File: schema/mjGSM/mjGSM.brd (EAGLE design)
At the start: 62 x 47 mm, 20 parts, among them Q1 16MHz, SW1 SPST, U1 ATMEGA328P-PU, X2 PWR

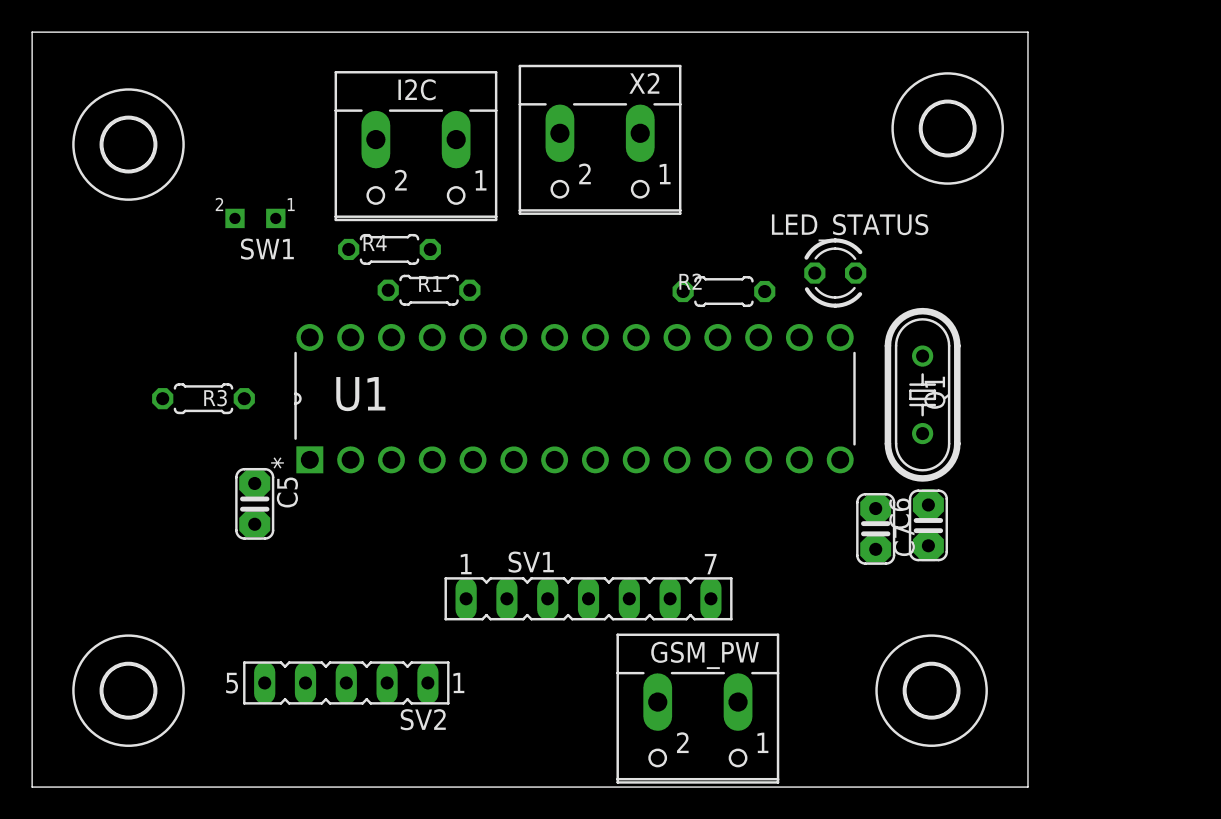
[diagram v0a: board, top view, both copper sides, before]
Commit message: mod
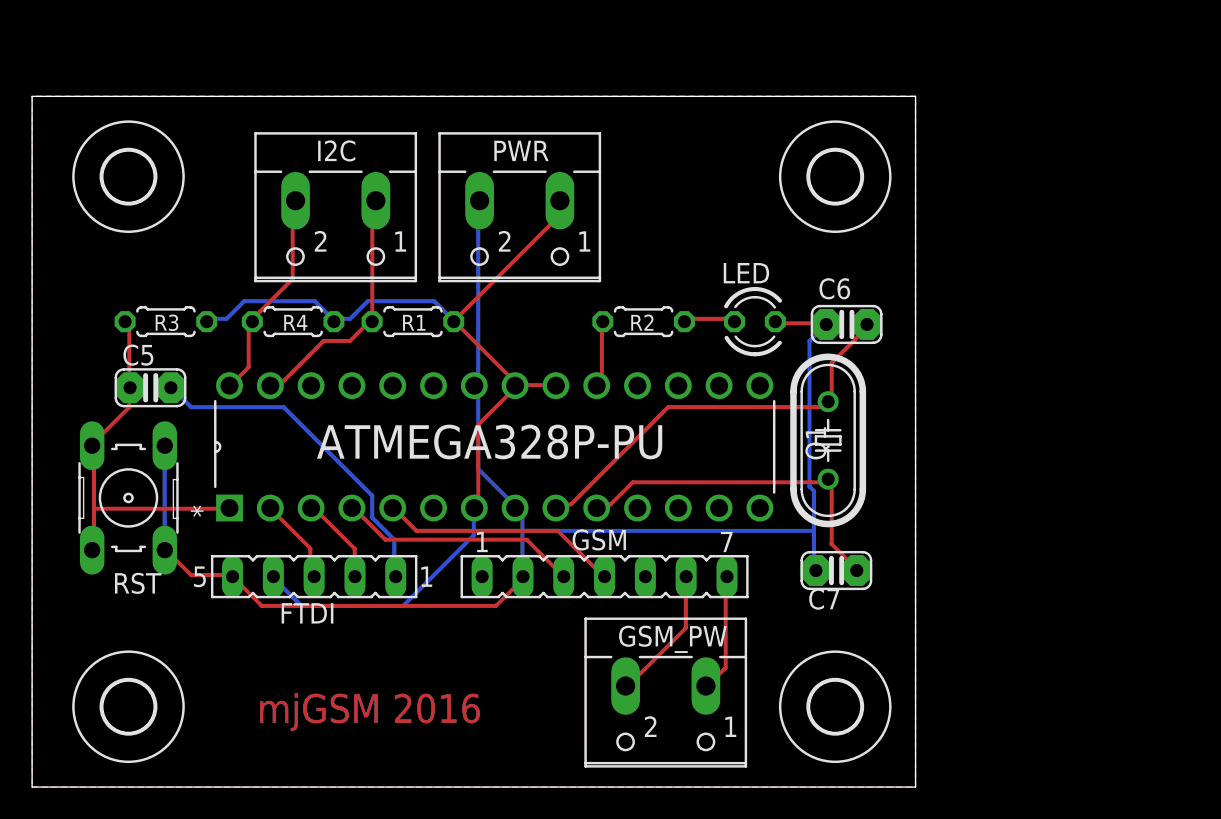
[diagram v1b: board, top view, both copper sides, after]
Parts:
- removed LED_STATUS: (no value), led:LED3MM
- removed SV1: GSM, con-lsta:FE07
- removed SV2: (no value), con-lsta:FE05-1
- removed SW1: SPST, gm-switches:SPST
- removed U1: ATMEGA328P-PU, Atmel_By_element14_Batch_1-00:DIP254P762X457-28
- removed X2: PWR, con-wago-500:W237-102
- added ATMEGA328P-PU: ATMEGA328P-PU, Atmel_By_element14_Batch_1-00:DIP254P762X457-28
- added FTDI: (no value), con-lsta:FE05-1
- added GSM: GSM, con-lsta:FE07
- added LED: (no value), led:LED3MM
- added PWR: PWR, con-wago-500:W237-102
- added RST: (no value), switch-omron:B3F-10XX
- moved C6 13.5 mm to (50.7, 28.8), turned to 0 degrees
- moved C5 9.72 mm to (7.37, 24.9), turned to 0 degrees
- moved H4 7.62 mm to (50.0, 38.0)
- moved R4 7.50 mm to (16.2, 29.0)
- moved Q1 6.53 mm to (49.6, 21.6), turned to 90 degrees
- moved I2C 6.28 mm to (18.9, 35.2)
- moved H3 6.08 mm to (50.0, 5.00)
- moved R2 5.34 mm to (38.1, 29.0)
- moved R3 5.34 mm to (8.33, 29.0), turned to 0 degrees
- moved C7 3.57 mm to (50.1, 13.5), turned to 0 degrees
- moved GSM_PW 2.24 mm to (39.5, 5.02)
- moved R1 2.20 mm to (23.7, 29.0)
- moved H2 2.00 mm to (6.00, 38.0)
- moved H1 1.00 mm to (6.00, 5.00)
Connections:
- net GND: now also ATMEGA328P-PU.22, ATMEGA328P-PU.8, FTDI.5, GSM.2, LED.K, PWR.2, RST.3, RST.4; no longer LED_STATUS.K, SV1.2, SV2.5, SW1.2, U1.22, U1.8, X2.2
- net GSM_RX: now also ATMEGA328P-PU.4, GSM.3; no longer SV1.3, U1.4
- net GSM_TX: now also ATMEGA328P-PU.5, GSM.4; no longer SV1.4, U1.5
- net N$1: now also LED.A; no longer LED_STATUS.A
- net N$10: now also GSM.7; no longer SV1.7
- net N$2: now also ATMEGA328P-PU.19; no longer U1.19
- net N$3: now also ATMEGA328P-PU.2, FTDI.3; no longer SV2.3, U1.2
- net N$4: now also ATMEGA328P-PU.3, FTDI.2; no longer SV2.2, U1.3
- net N$5: now also ATMEGA328P-PU.1, RST.1, RST.2; no longer SW1.1, U1.1
- net N$6: now also ATMEGA328P-PU.9; no longer U1.9
- net N$7: now also FTDI.1; no longer SV2.1
- net N$8: now also ATMEGA328P-PU.10; no longer U1.10
- net N$9: now also GSM.6; no longer SV1.6
- net SCL: now also ATMEGA328P-PU.28; no longer U1.28
- net SDA: now also ATMEGA328P-PU.27; no longer U1.27
- net VCC: now also ATMEGA328P-PU.20, ATMEGA328P-PU.21, ATMEGA328P-PU.7, FTDI.4, PWR.1; no longer SV2.4, U1.20, U1.21, U1.7, X2.1
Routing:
- net GND: track 0.00 -> 93.2 mm
- net VCC: track 0.00 -> 61.4 mm
- net N$6: track 0.00 -> 25.6 mm
- net N$5: track 0.00 -> 23.9 mm
- net N$8: track 0.00 -> 21.7 mm
- net N$7: track 0.00 -> 21.0 mm
- net SDA: track 0.00 -> 15.6 mm
- net GSM_RX: track 0.00 -> 14.9 mm
- net GSM_TX: track 0.00 -> 14.9 mm
- net SCL: track 0.00 -> 13.3 mm
- net N$9: track 0.00 -> 8.44 mm
- net N$10: track 0.00 -> 7.38 mm
- net N$4: track 0.00 -> 5.49 mm
- net N$3: track 0.00 -> 5.45 mm
- net N$2: track 0.00 -> 4.14 mm
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- added copper zone on layer 1, net N$11
- added copper zone on layer 16, net N$12
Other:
- board size 62 x 47 mm -> 55 x 43 mm
- board text added: "mjGSM 2016"

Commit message: mod
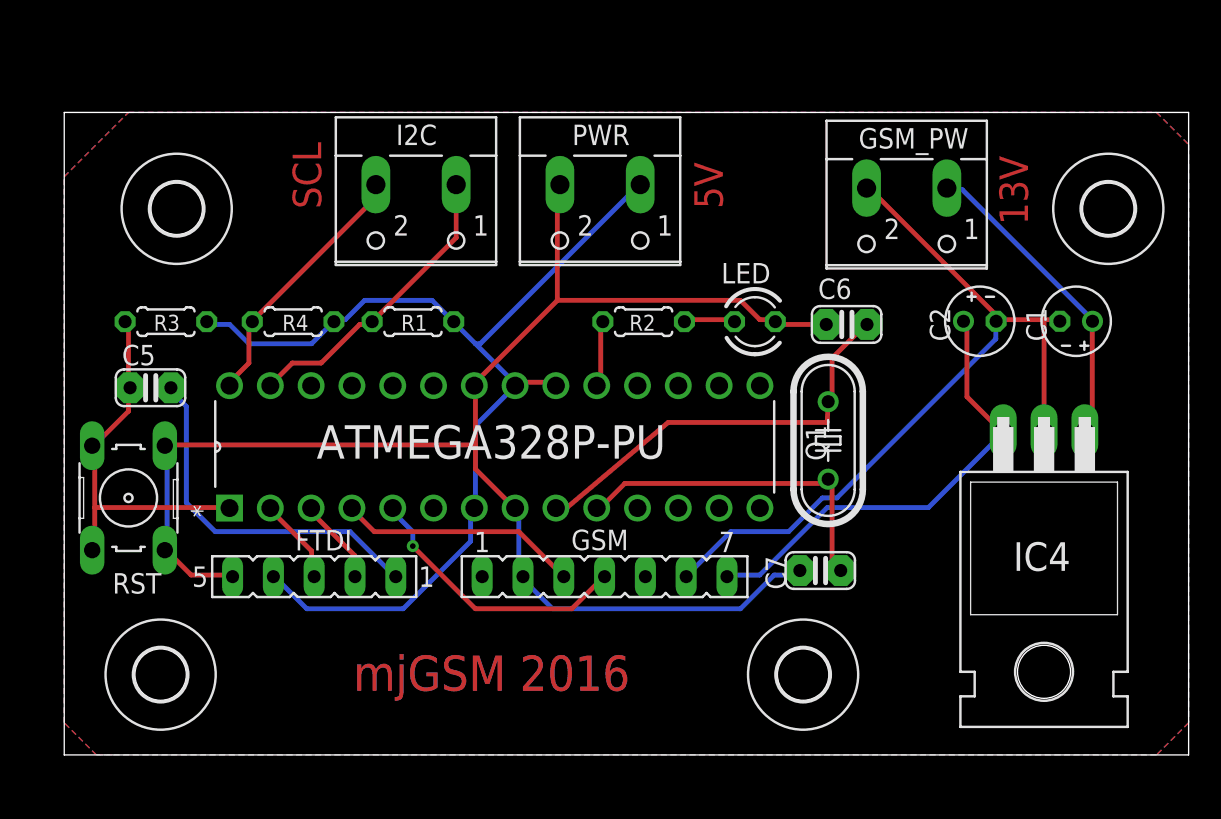
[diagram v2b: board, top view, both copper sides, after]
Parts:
- added C1, C2: 100nF, rcl:E2-4
- added IC4: 7805T, linear:TO220H
- GSM_PW: value GND -> (none)
- PWR: value PWR -> (none)
- moved GSM_PW 34.4 mm to (54.5, 36.0)
- moved H4 17.1 mm to (67.0, 36.0)
- moved I2C 5.10 mm to (23.9, 36.2)
- moved PWR 5.10 mm to (35.4, 36.2)
- moved H2 3.61 mm to (9.00, 36.0)
- moved H1 2.83 mm to (8.00, 7.00)
- moved H3 2.83 mm to (48.0, 7.00)
- moved C7 1.00 mm to (49.1, 13.5)
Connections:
- removed net N$10: GSM.7, GSM_PW.1
- removed net N$9: GSM.6, GSM_PW.2
- new net 13V: C1.+, GSM_PW.1, IC4.1
- new net GSM5V: C2.+, GSM.7, IC4.3
- new net GSMGND: C1.-, C2.-, GSM.6, GSM_PW.2, IC4.2
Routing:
- net GSMGND: track 0.00 -> 49.2 mm
- net GSM5V: track 0.00 -> 28.9 mm
- net 13V: track 0.00 -> 19.6 mm
- net N$9: track 8.44 -> 0.00 mm
- net N$10: track 7.38 -> 0.00 mm
- net VCC: track 61.4 -> 65.9 mm
- net SDA: track 15.6 -> 18.7 mm
- net SCL: track 13.3 -> 16.3 mm
- net GSM_TX: track 14.9 -> 17.2 mm, vias 0 -> 1
- net GND: track 93.2 -> 95.4 mm
- net N$7: track 21.0 -> 22.5 mm
- net N$6: track 25.6 -> 26.1 mm
- added copper zone on layer 16, net N$10
- added copper zone on layer 1, net N$9
- removed copper zone on layer 1, net N$11
- removed copper zone on layer 16, net N$12
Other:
- board size 55 x 43 mm -> 70 x 40 mm
- board text added: "13V"
- board text added: "5V"
- board text added: "SCL"
